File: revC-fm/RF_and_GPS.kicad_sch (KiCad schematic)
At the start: 8 parts, among them J8 SMPM-PS-P-HG-ST-EM-1, J9 SMPM-PS-P-HG-ST-EM-1, U21 RFM98PW, U22 S1216V8, U23 RFM9xBreakout

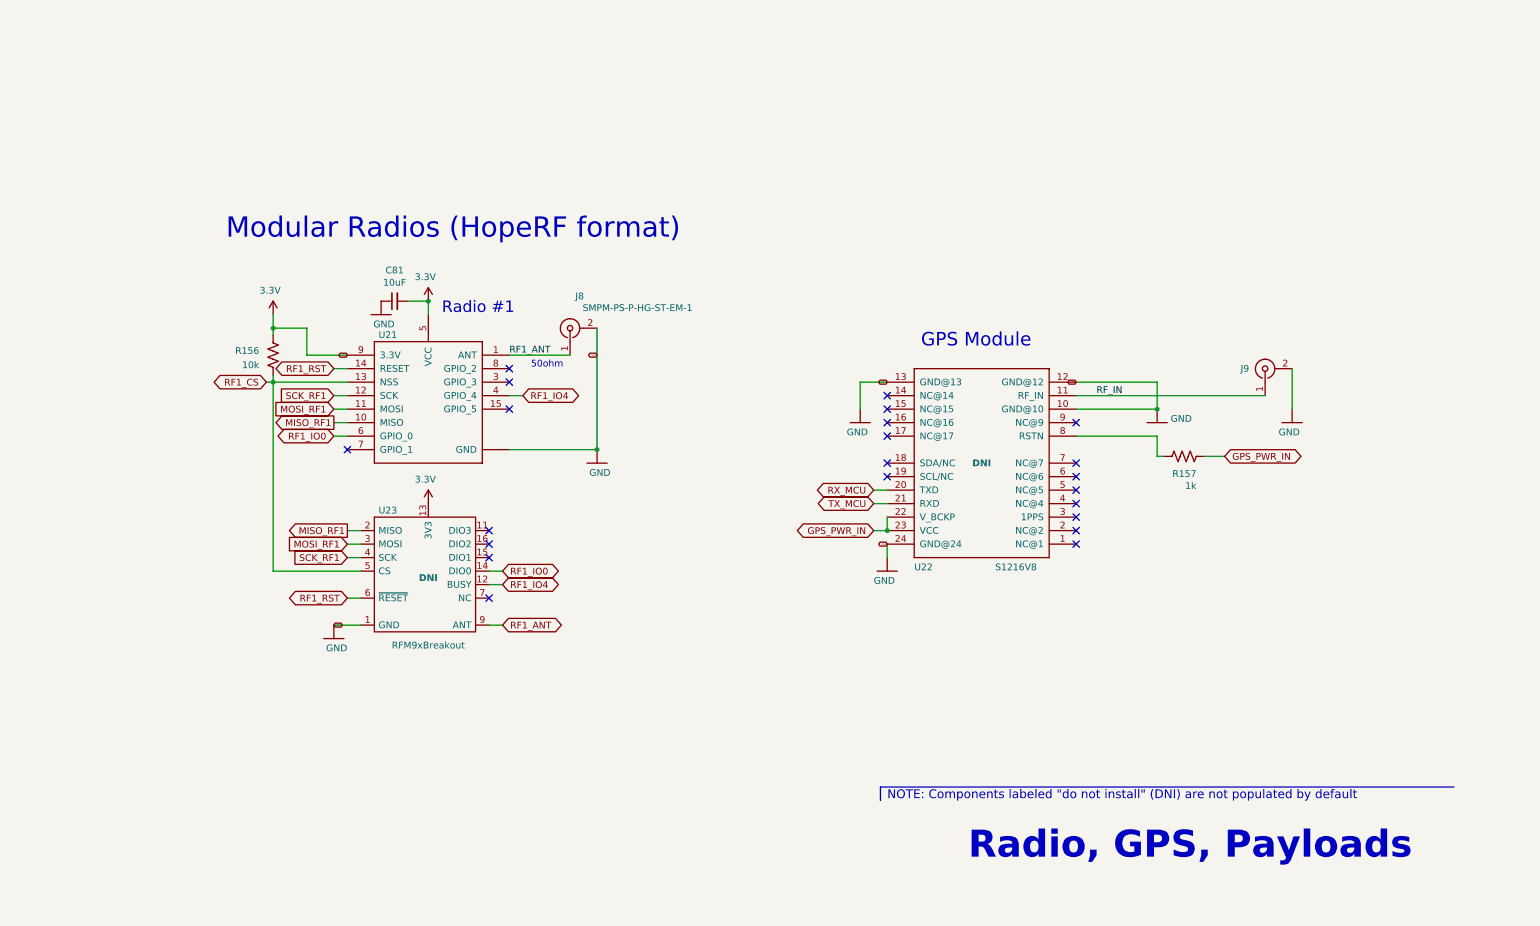
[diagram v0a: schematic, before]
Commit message: working revC
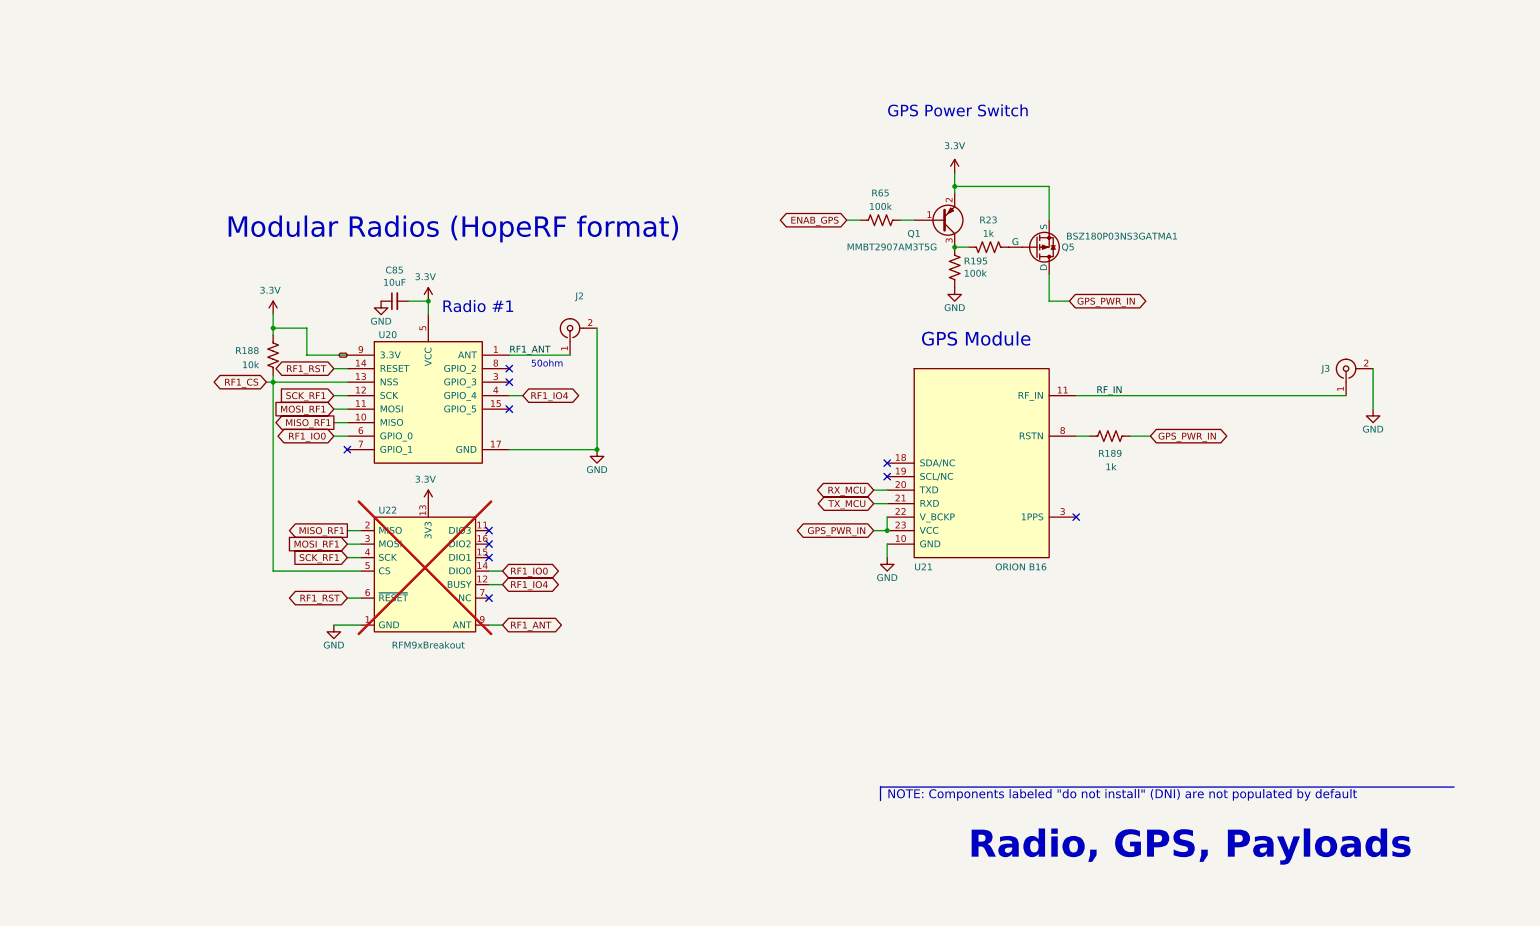
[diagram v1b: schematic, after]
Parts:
- added Q1: MMBT2907AM3T5G, Package_TO_SOT_SMD:SOT-723, symbol Device:Q_PNP_BEC
- added Q5: BSZ180P03NS3GATMA1, SierraLobo:PG-TSDSON-8_3.3x3.3mm, symbol SierraLobo:BSZ086
- added R195, R65: 100k, Resistor_SMD:R_0603_1608Metric, symbol Device:R_US
- added R23: 1k, Resistor_SMD:R_0603_1608Metric, symbol Device:R_US
- J2: renamed from J8; footprint mainboard-SLI:J-MOLEX-SMPM-073300-003X_no_Back -> SierraLobo:SMPM-073300-003X_no_Back
- J3: renamed from J9; footprint mainboard-SLI:J-MOLEX-SMPM-073300-003X_no_Back -> SierraLobo:SMPM-073300-003X_no_Back
- U20: renamed from U21; footprint mainboard:RFM95PW -> SierraLobo:RFM95PW; symbol mainboard:RFM98PW -> SierraLobo:RFM98PW; Flight RFM98PW -> (none); Manufacturer_Name HopeRF -> (none); Manufacturer_Part_Number RFM98PW -> (none); Proto RFM98PW -> (none)
- U21: renamed from U22; value S1216V8 -> ORION B16; footprint mainboard:S1216_24PIN_PACKAGE -> SierraLobo:S1216_24PIN_PACKAGE; symbol mainboard:S1216V8 -> SierraLobo:S1216V8; DNI DNI -> (none)
- U22: renamed from U23; symbol mainboard:RFM9xBreakout -> SierraLobo:RFM9xBreakout; DNI DNI -> (none); now not fitted
- renumbered C81 to C85, R156 to R188, R157 to R189
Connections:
- net 3.3V: now also Q1.2 (E), Q5.1 (S)
- net GND: now also R195.2
- net GPS_PWR_IN: now also Q5.5 (D)
- net at U21.1 (NC): now also U21.14 (NC), U21.15 (NC), U21.16 (NC), U21.17 (NC), U21.2 (NC), U21.4 (NC), U21.5 (NC), U21.6 (NC), U21.7 (NC), U21.9 (NC)
- new net: Q5.4 (G), R23.1
- new net: Q1.3 (C), R195.1, R23.2
- new net: Q1.1 (B), R65.2
- new net ENAB_GPS: R65.1
- no-connect marks 22 -> 11
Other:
- note added: "GPS Power Switch"
- moved on the sheet: J3, R189

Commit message: routing fm
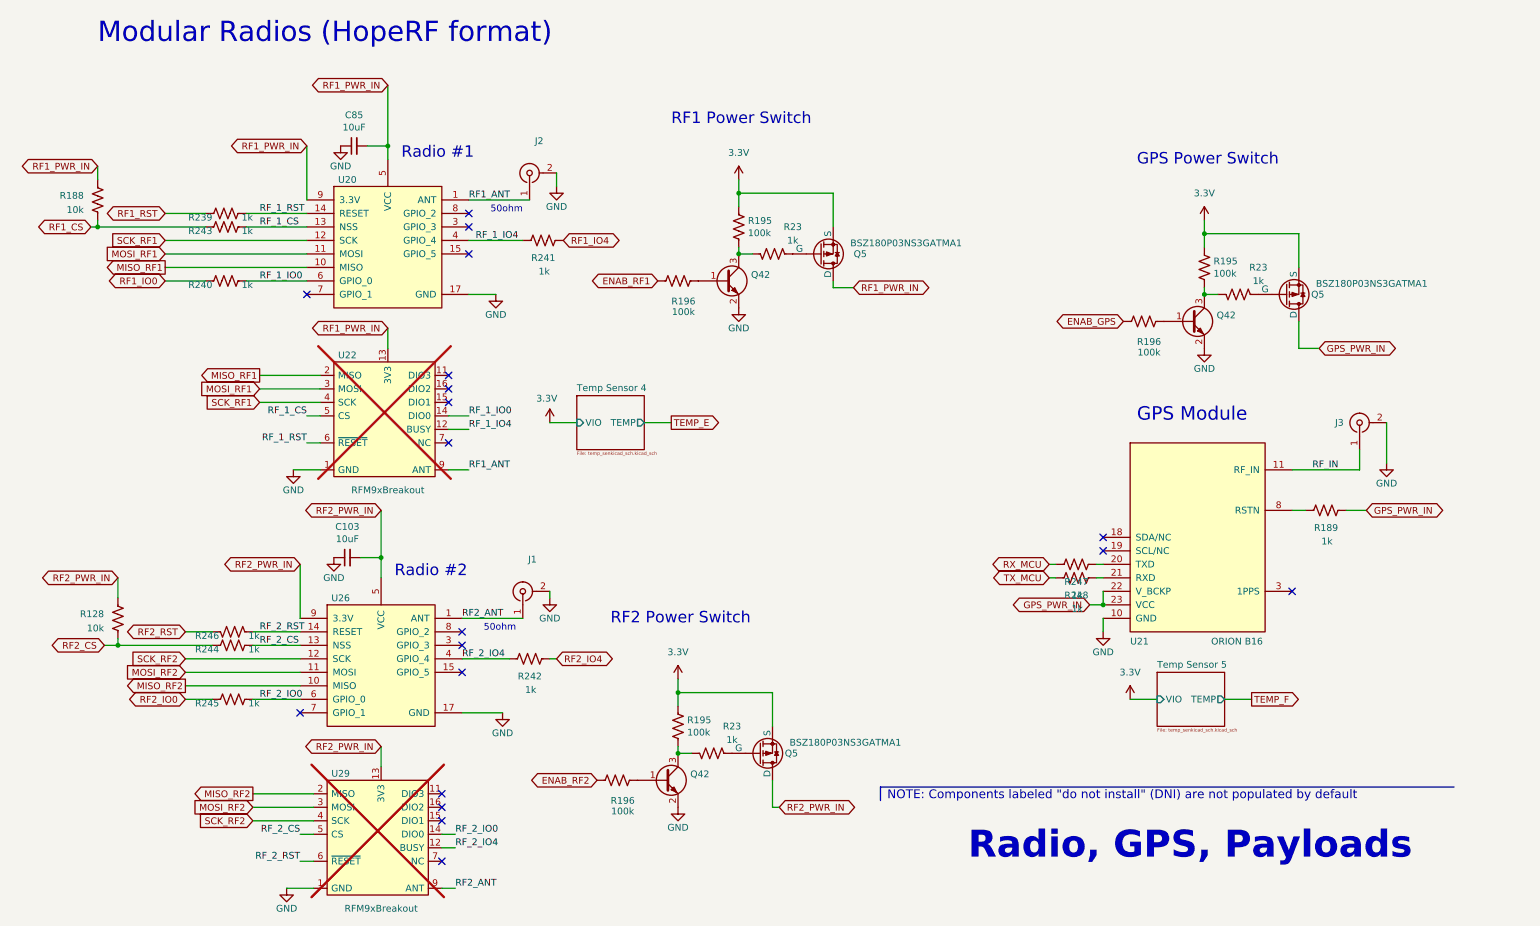
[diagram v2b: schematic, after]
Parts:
- removed Q1: MMBT2907AM3T5G, Package_TO_SOT_SMD:SOT-723, symbol Device:Q_PNP_BEC
- removed R65: 100k, Resistor_SMD:R_0603_1608Metric, symbol Device:R_US
- added C103: 10uF, Capacitor_SMD:C_0805_2012Metric, symbol Device:C_Small
- added J1: SMPM-PS-P-HG-ST-EM-1, SierraLobo:SMPM-073300-003X_no_Back, symbol mainboard-rescue:Conn_Coaxial-Connector-mainboard-rescue
- added Q42 (x3): ~, Package_TO_SOT_SMD:SOT-323_SC-70, symbol Device:Q_NPN_BEC
- added Q5 (x2): BSZ180P03NS3GATMA1, SierraLobo:PG-TSDSON-8_3.3x3.3mm, symbol SierraLobo:BSZ086
- added R128: 10k, Resistor_SMD:R_0603_1608Metric, symbol Device:R_US
- added R195 (x2), R196 (x3): 100k, Resistor_SMD:R_0603_1608Metric, symbol Device:R_US
- added R23 (x2), R239, R240, R241, R242, R243, R244, R245, R246, R247, R248: 1k, Resistor_SMD:R_0603_1608Metric, symbol Device:R_US
- added U26: RFM98PW, SierraLobo:RFM95PW, symbol SierraLobo:RFM98PW
- added U29: RFM9xBreakout, RF_Module:HOPERF_RFM9XW_SMD, symbol SierraLobo:RFM9xBreakout
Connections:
- net 3.3V: now also R195.1, Q5.1 (S), Q5.1 (S), R195.1, R195.1; no longer C85.2, R188.1, U20.5 (VCC), U20.9 (3.3V), U22.13 (3V3)
- net ENAB_GPS: now also R196.2
- net GND: now also C103.1, J1.2 (Ext), Q42.2 (E), Q42.2 (E), Q42.2 (E), U26.16 (GND), U26.17 (GND), U26.2 (GND), U29.1 (GND), U29.10 (GND), U29.8 (GND); no longer R195.2
- net RF1_CS: now also R243.1; no longer U20.13 (NSS), U22.5 (CS)
- net RF1_IO0: now also R240.1; no longer U20.6 (GPIO_0), U22.14 (DIO0)
- net RF1_IO4: now also R241.2; no longer U20.4 (GPIO_4), U22.12 (BUSY)
- net RF1_RST: now also R239.1; no longer U20.14 (RESET), U22.6 (~{RESET})
- net RX_MCU: now also R247.1; no longer U21.20 (TXD)
- net TX_MCU: now also R248.1; no longer U21.21 (RXD)
- net at R23.2: now also R195.2, Q42.3 (C); no longer R195.1
- new net: R247.2, U21.20 (TXD)
- new net: R248.2, U21.21 (RXD)
- new net: Q42.1 (B), R196.1 (x3)
- new net: Q42.3 (C), R195.2, R23.2 (x2)
- new net: Q5.4 (G), R23.1 (x2)
- new net ENAB_RF1: R196.2
- new net ENAB_RF2: R196.2
- new net MISO_RF2: U26.10 (MISO), U29.2 (MISO)
- new net MOSI_RF2: U26.11 (MOSI), U29.3 (MOSI)
- new net RF1_PWR_IN: C85.2, Q5.5 (D), R188.1, U20.5 (VCC), U20.9 (3.3V), U22.13 (3V3)
- new net RF2_ANT: J1.1 (In), U26.1 (ANT), U29.9 (ANT)
- new net RF2_CS: R128.2, R244.1
- new net RF2_IO0: R245.1
- new net RF2_IO4: R242.2
- new net RF2_PWR_IN: C103.2, Q5.5 (D), R128.1, U26.5 (VCC), U26.9 (3.3V), U29.13 (3V3)
- new net RF2_RST: R246.1
- new net RF_1_CS: R243.2, U20.13 (NSS), U22.5 (CS)
- new net RF_1_IO0: R240.2, U20.6 (GPIO_0), U22.14 (DIO0)
- new net RF_1_IO4: R241.1, U20.4 (GPIO_4), U22.12 (BUSY)
- new net RF_1_RST: R239.2, U20.14 (RESET), U22.6 (~{RESET})
- new net RF_2_CS: R244.2, U26.13 (NSS), U29.5 (CS)
- new net RF_2_IO0: R245.2, U26.6 (GPIO_0), U29.14 (DIO0)
- new net RF_2_IO4: R242.1, U26.4 (GPIO_4), U29.12 (BUSY)
- new net RF_2_RST: R246.2, U26.14 (RESET), U29.6 (~{RESET})
- new net SCK_RF2: U26.12 (SCK), U29.4 (SCK)
- no-connect marks 11 -> 19
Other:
- added sheet Temp Sensor 4 (temp_senkicad_sch.kicad_sch)
- added sheet Temp Sensor 5 (temp_senkicad_sch.kicad_sch)
- note added: "RF1 Power Switch"
- note added: "RF2 Power Switch"
- note added: "Radio #2"
- moved on the sheet: C85, J2, J3, Q5, R188, R189, R195, R23, U20, U21, U22
